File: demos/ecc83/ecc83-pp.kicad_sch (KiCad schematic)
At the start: 15 parts, among them P1 IN, P2 OUT, P3 POWER, P4 CONN_2, P5 MOUNTING_HOLE, P6 MOUNTING_HOLE, P7 MOUNTING_HOLE, P8 MOUNTING_HOLE, U1 ECC83

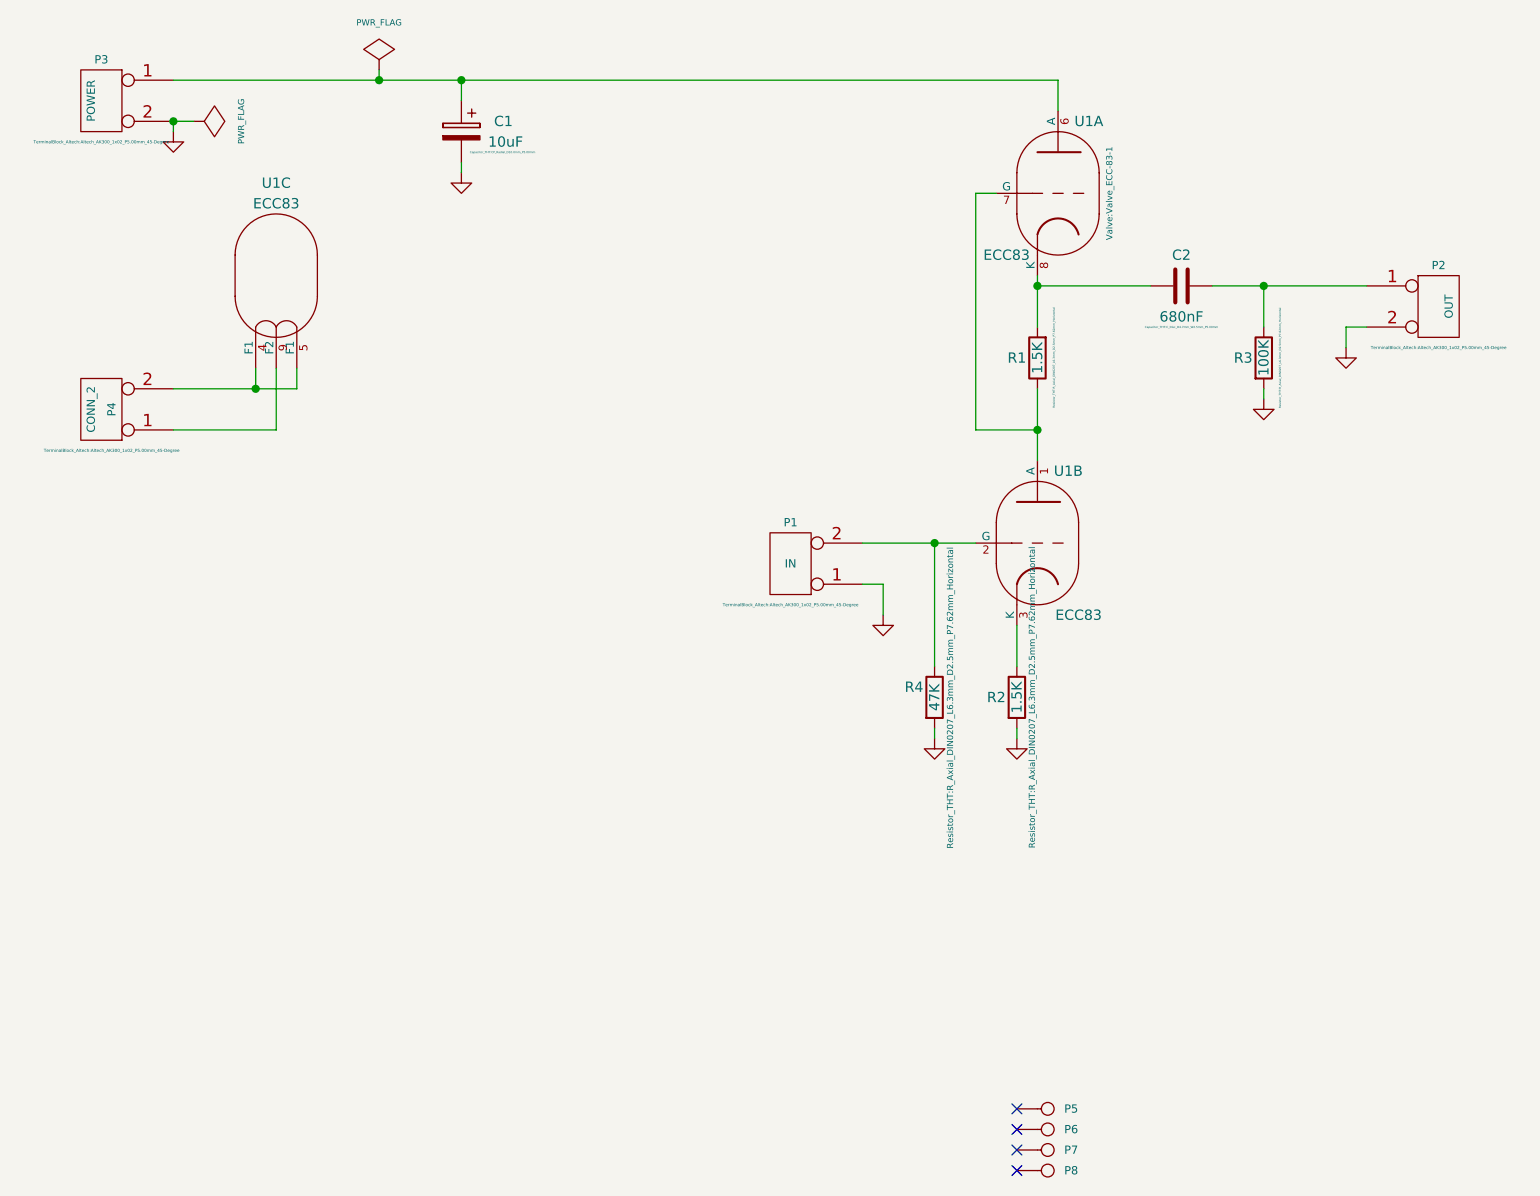
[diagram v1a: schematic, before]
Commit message: Demos update
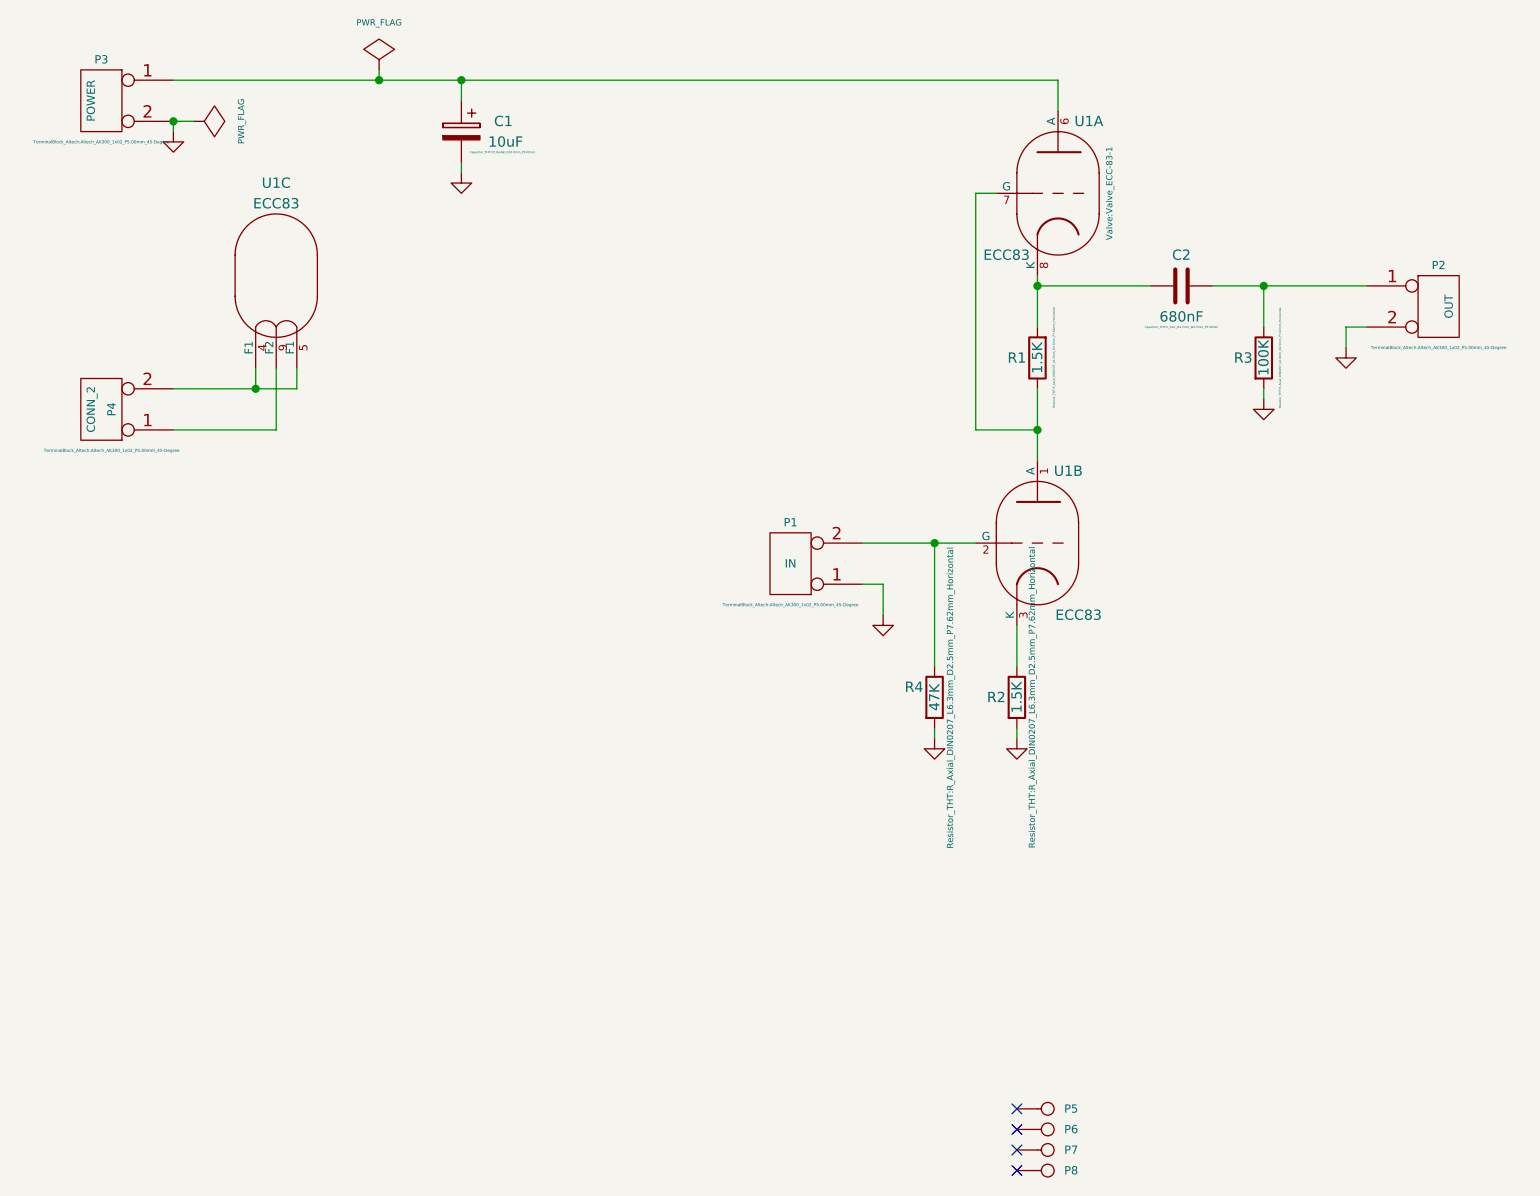
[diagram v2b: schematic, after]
